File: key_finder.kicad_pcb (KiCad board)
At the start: 2 copper layers, 20 x 14 mm, 18 parts, among them U1 NRF52832, X1 32MHz, X2 32.768kHz

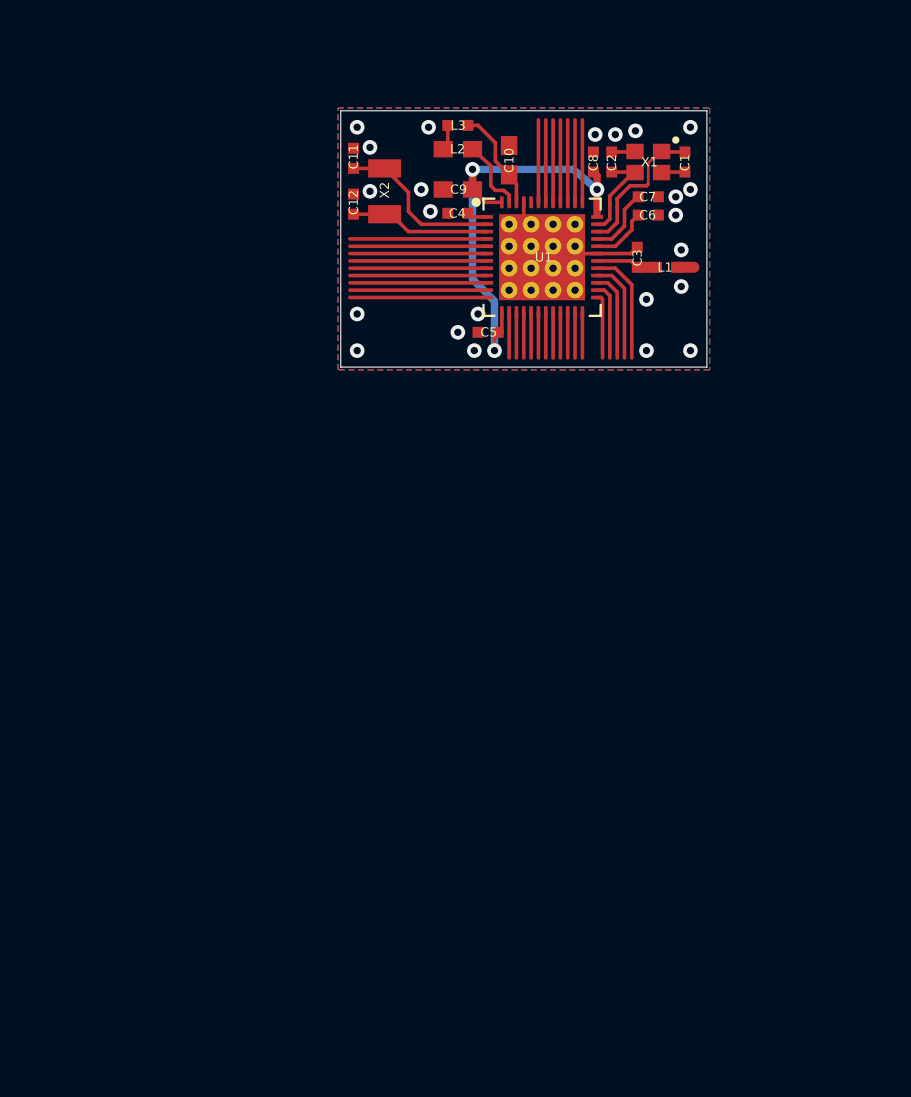
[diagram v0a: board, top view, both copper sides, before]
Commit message: end of shematic
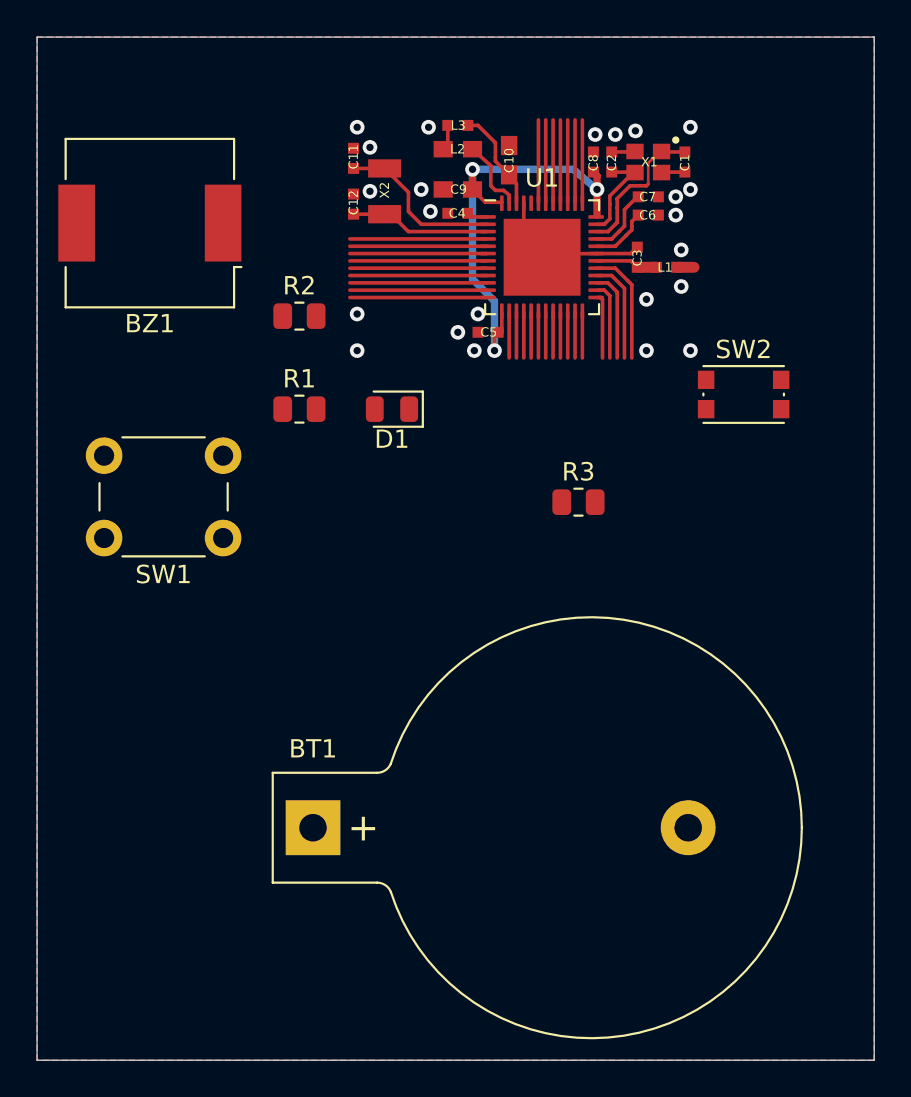
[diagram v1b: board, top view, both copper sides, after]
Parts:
- added BT1: Battery, Battery:BatteryHolder_Keystone_103_1x20mm, F.Cu at (137.0, 137.2)
- added BZ1: Buzzer, Buzzer_Beeper:Buzzer_CUI_CPT-9019S-SMT, F.Cu at (128.1, 104.1)
- added D1: LED, LED_SMD:LED_0805_2012Metric, F.Cu at (141.3, 114.3)
- added R1: 330, Resistor_SMD:R_0805_2012Metric, F.Cu at (136.2, 114.3)
- added R2: 10k, Resistor_SMD:R_0805_2012Metric, F.Cu at (136.2, 109.2)
- added R3: 10k, Resistor_SMD:R_0805_2012Metric, F.Cu at (151.5, 119.4)
- added SW1: SW_Push, Button_Switch_THT:SW_PUSH_6mm_H7.3mm, F.Cu at (132.1, 121.3)
- added SW2: SW_Push, Button_Switch_SMD:SW_Push_1P1T_NO_CK_KMR2, F.Cu at (160.5, 113.5)
- U1: footprint QFN40P600X600X90-48_N -> Package_DFN_QFN:QFN-48-1EP_6x6mm_P0.4mm_EP4.2x4.2mm
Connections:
- net P0.02 renamed /P0.02
- net P0.03 renamed /P0.03
- net P0.05 renamed /P0.05
- net P0.07 renamed /P0.07
- net P0.08 renamed /P0.08
- net P0.09 renamed /P0.09
- net P0.11 renamed /P0.11
- net P0.12 renamed /P0.12
- net P0.13 renamed /P0.13
- net P0.14 renamed /P0.14
- net P0.15 renamed /P0.15
- net P0.16 renamed /P0.16
- net P0.17 renamed /P0.17
- net P0.18/SWO renamed /P0.18/SWO
- net P0.19 renamed /P0.19
- net P0.20 renamed /P0.20
- net P0.22 renamed /P0.22
- net P0.23 renamed /P0.23
- net P0.24 renamed /P0.24
- net P0.25 renamed /P0.25
- net P0.26 renamed /P0.26
- net P0.27 renamed /P0.27
- net P0.28 renamed /P0.28
- net P0.29 renamed /P0.29
- net P0.30 renamed /P0.30
- net P0.31 renamed /P0.31
- net SWDCLK renamed /SWDCLK
- net SWDIO renamed /SWDIO
- U1 pad 1: DEC1 -> /DEC1
- U1 pad 12: P0.10 -> /P0.10
- U1 pad 13: VDD_P3V3 -> VCC
- U1 pad 2: P0.00/XL1 -> /P0.00/XL1
- U1 pad 24: P0.21/RESET -> /P0.21/RESET
- U1 pad 3: P0.01/XL2 -> /P0.01/XL2
- U1 pad 30: ANT -> Net-(U1-ANT@30)
- U1 pad 32: DEC2 -> /DEC2
- U1 pad 33: DEC3 -> /DEC3
- U1 pad 34: X1 -> Net-(U1-XC1@34)
- U1 pad 35: N$3 -> Net-(U1-XC2@35)
- U1 pad 36: VDD_P3V3 -> VCC
- U1 pad 44: (no net) -> unconnected-(U1-N.C.@44-Pad44)
- U1 pad 46: DEC4 -> /DEC4
- U1 pad 47: N$4 -> Net-(U1-DCC@47)
- U1 pad 48: VDD_P3V3 -> VCC
- U1 pad 6: P0.04 -> /P0.04
- U1 pad 8: P0.06 -> /P0.06
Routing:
- net P0.10: track 7.50 -> 0.00 mm
- net P0.06: track 7.50 -> 0.00 mm
- net P0.04: track 7.50 -> 0.00 mm
- net /P0.10: track 0.00 -> 7.50 mm
- net /P0.06: track 0.00 -> 7.50 mm
- net /P0.04: track 0.00 -> 7.50 mm
- net P0.21/RESET: track 2.50 -> 0.00 mm
- net /P0.21/RESET: track 0.00 -> 2.50 mm
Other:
- board size 20 x 14 mm -> 45.7 x 55.9 mm
